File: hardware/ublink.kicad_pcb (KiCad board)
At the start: 2 copper layers, 67 x 54.5 mm, 62 parts, among them J1 USB_B_Micro, J2 AC1, J3 5V Trafo, J4 Screw_Terminal_01x02, J5 Screw_Terminal_01x02, J7 Screw_Terminal_01x02, J8 JTAG/UART, J9 Screw_Terminal_01x02, Q1 STN3NF06L, Q2 RU6099, Q3 RU6099, Q4 RU6099, Q5 RU6099, Q6 NMOS, SW1 SW_Push, SW2 SW_Push, SW3 JUC-31F, U1 3.3V3 Regul, U2 CH340G, U3 HF115F_005-1ZS3, U4 ESP32-WROOM-32U, U5 EL817S, U6 EL817S, U7 EL817S, U8 EL817S, Y1 12Mhz

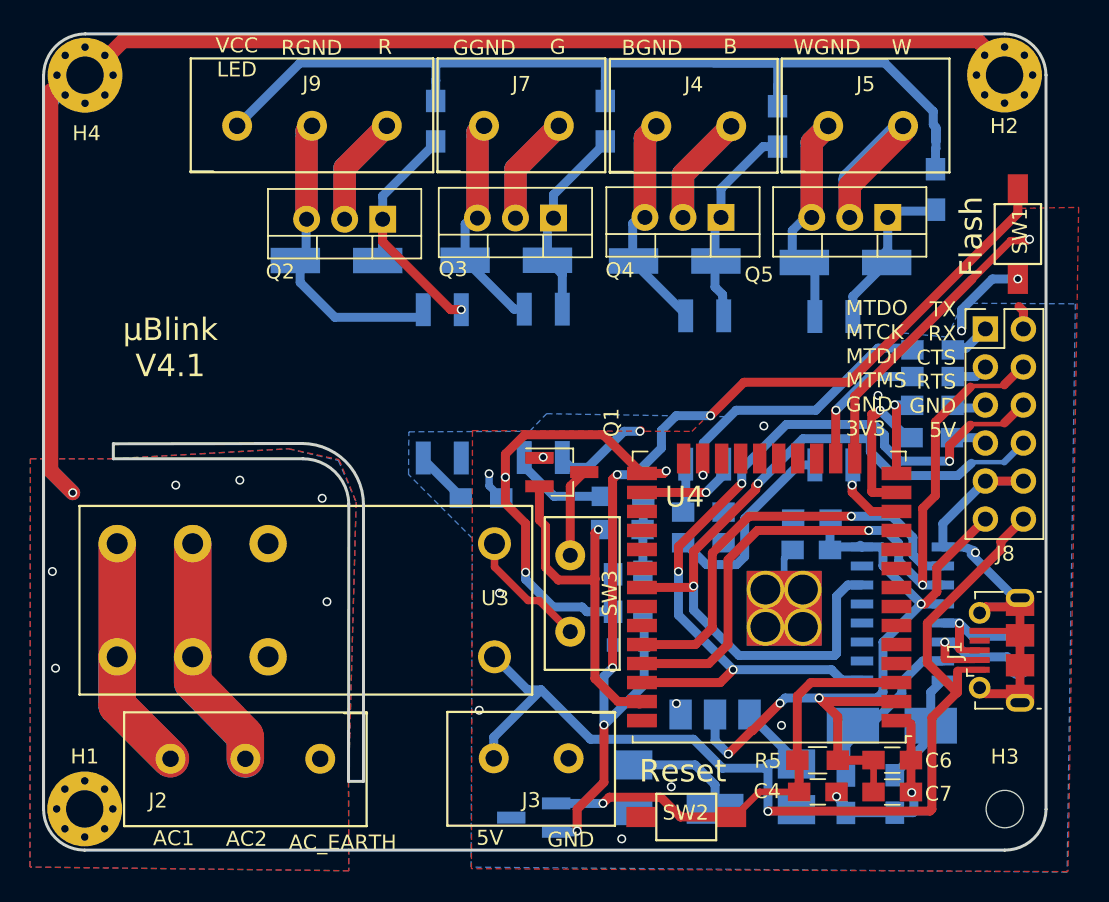
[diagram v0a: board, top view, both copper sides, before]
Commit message: Initial firmware
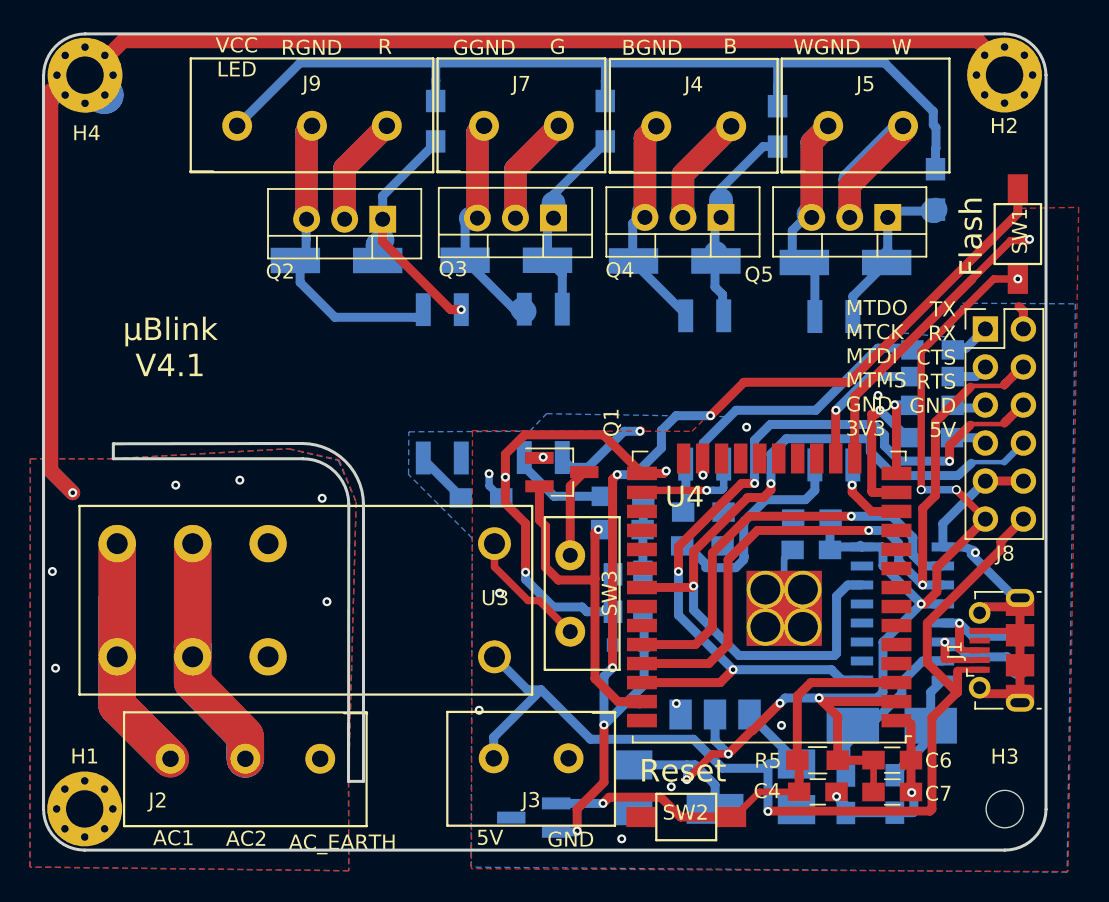
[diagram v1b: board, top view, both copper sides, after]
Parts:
- moved R11 0.22 mm to (154.1, 122.8)
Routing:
- net 3V3: track 70.5 -> 91.5 mm, vias 6 -> 8
- net /LED_VCC: track 66.6 -> 61.5 mm
- net AC2: track 31.7 -> 35.5 mm
- net CTS: track 55.7 -> 57.8 mm
- net RTS: track 51.3 -> 53.0 mm
- net /B_GATE: track 15.8 -> 17.5 mm
- net Net-(C3-Pad1): track 7.88 -> 9.54 mm
- net /R_GATE: track 18.8 -> 20.3 mm
- net AC_SAFE: track 121.9 -> 123.4 mm
- net AC1: track 31.3 -> 32.8 mm
- net /USB_D-: track 8.23 -> 9.65 mm
- net B_CTRL: track 6.66 -> 7.89 mm
- net EN: track 31.2 -> 32.4 mm
- net Net-(R11-Pad2): track 13.8 -> 14.9 mm
- net RX: track 47.9 -> 48.9 mm
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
